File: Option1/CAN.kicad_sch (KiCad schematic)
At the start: 6 parts, among them U301 TJA1051T-3

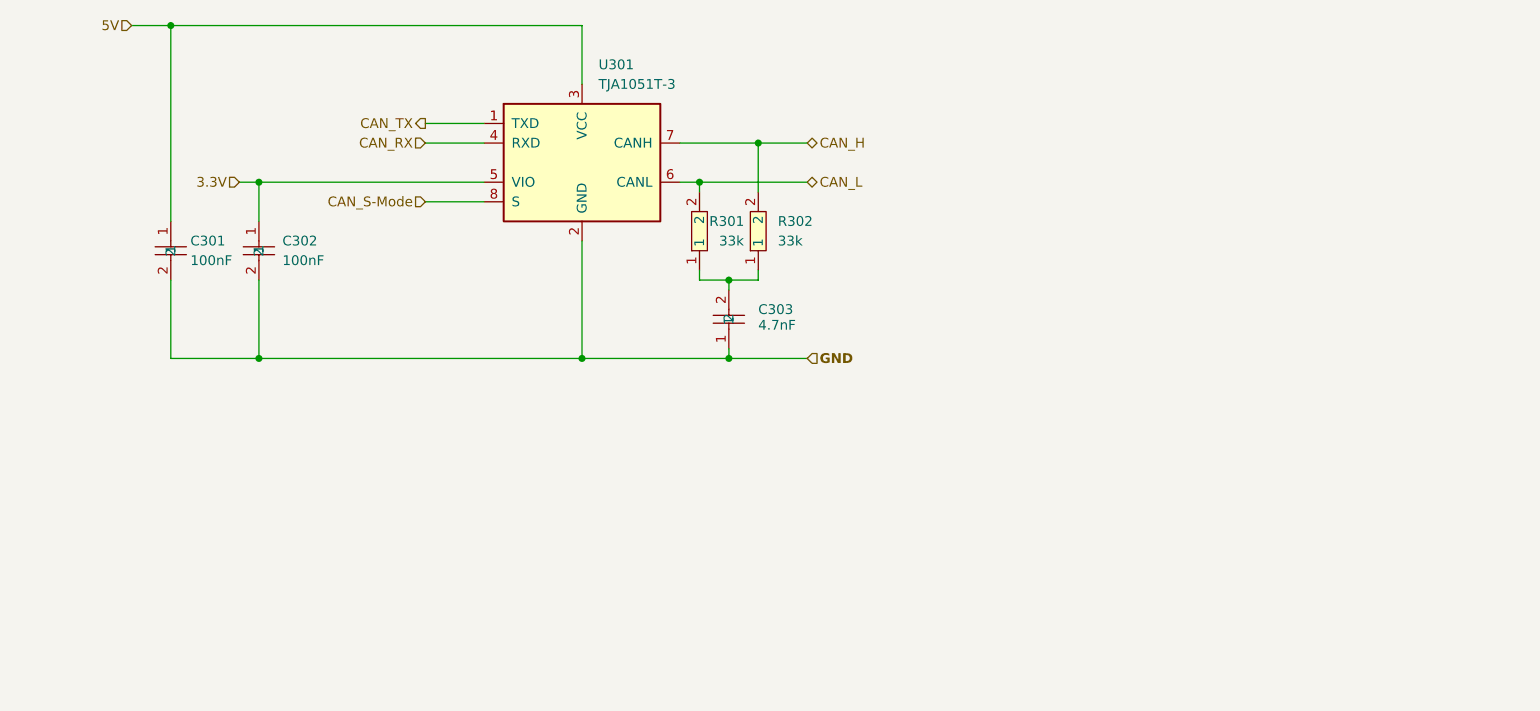
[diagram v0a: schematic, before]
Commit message: Erste issues eingearbeitet
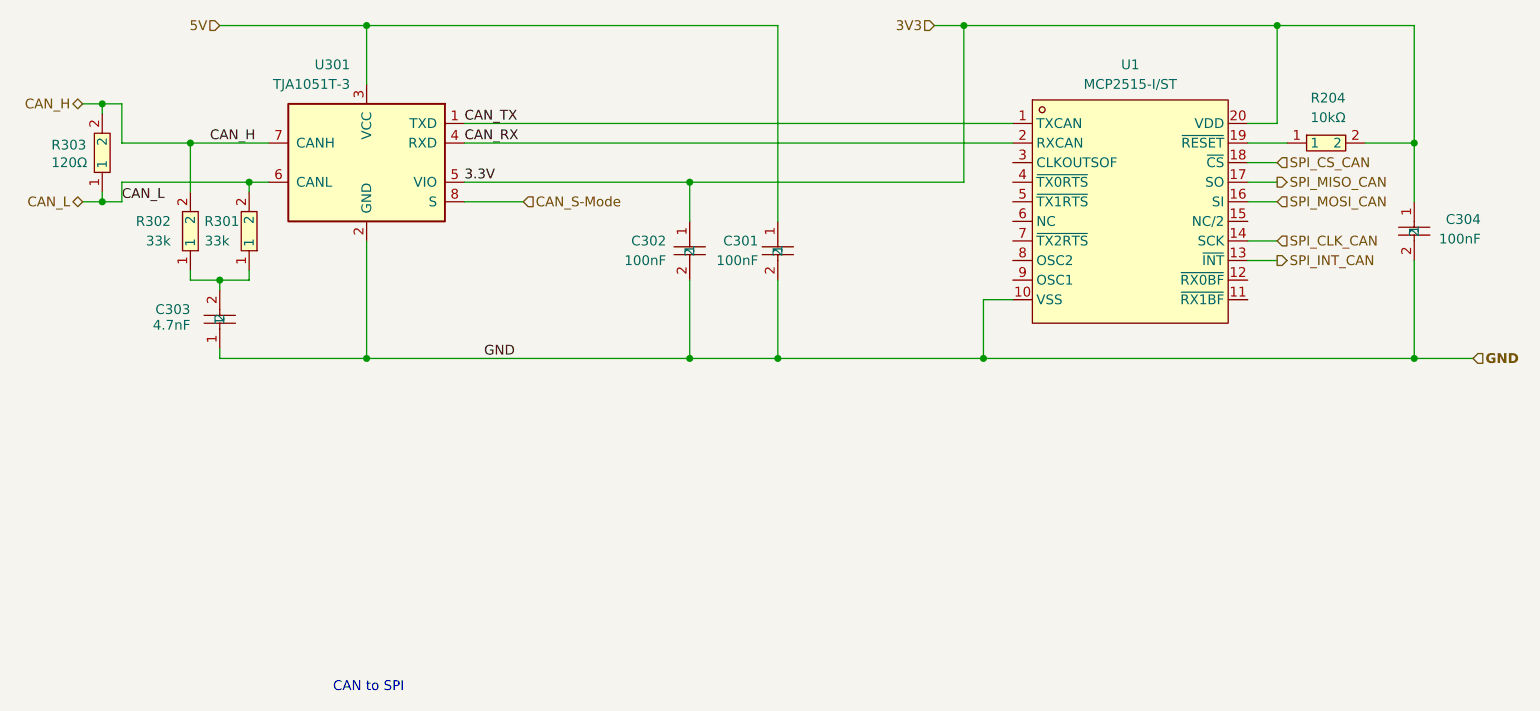
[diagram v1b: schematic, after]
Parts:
- added C304: 100nF, easyeda2kicad:C0603, symbol easyeda2kicad:CL10B104KA8NNNC
- added R204: 10kΩ, easyeda2kicad:R0603, symbol EasyEda2KiCad:0603WAF1002T5E
- added R303: 120Ω, easyeda2kicad:R0603, symbol EasyEda2KiCad:0603WAF1200T5E
- added U1: MCP2515-I/ST, easyeda2kicad:TSSOP-20_L6.5-W4.4-P0.65-LS6.4-BL, symbol EasyEda2KiCad:MCP2515-I_ST
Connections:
- net CAN_H: now also R303.2
- net CAN_L: now also R303.1
- net CAN_RX: now also U1.2 (RXCAN)
- net CAN_TX: now also U1.1 (TXCAN)
- net GND: now also C304.2, U1.10 (VSS)
- net 3.3V renamed 3V3
- net 3V3: now also C304.1, R204.2, U1.20 (VDD)
- new net: R204.1, U1.19 (~{RESET})
- new net SPI_CLK_CAN: U1.14 (SCK)
- new net SPI_CS_CAN: U1.18 (~{CS})
- new net SPI_INT_CAN: U1.13 (~{INT})
- new net SPI_MISO_CAN: U1.17 (SO)
- new net SPI_MOSI_CAN: U1.16 (SI)
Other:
- note added: "CAN to SPI"
- moved on the sheet: C301, C302, C303, R301, R302, U301
